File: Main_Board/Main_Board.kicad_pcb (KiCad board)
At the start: 2 copper layers, 3 parts, among them U1 TCR2EF33_LMCT

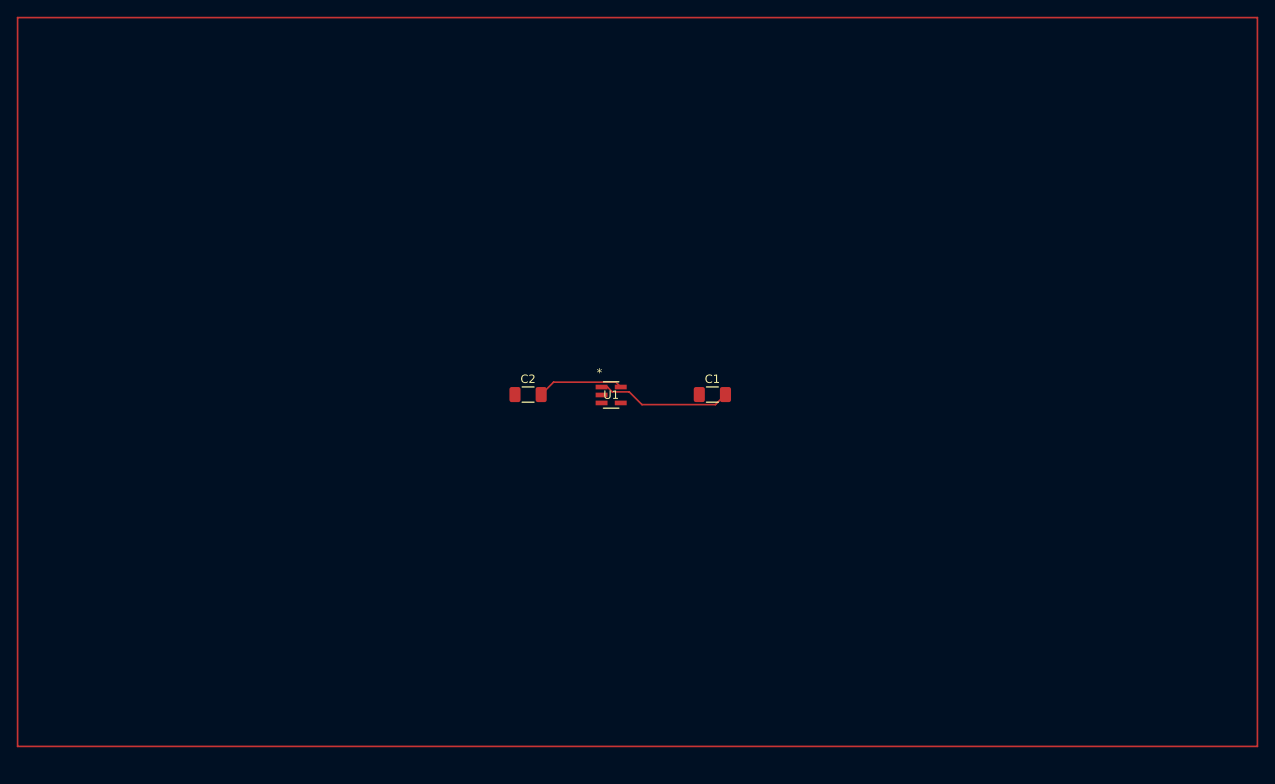
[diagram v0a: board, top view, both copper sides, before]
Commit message: Main board
The schematic is done, tho I have some concerns...
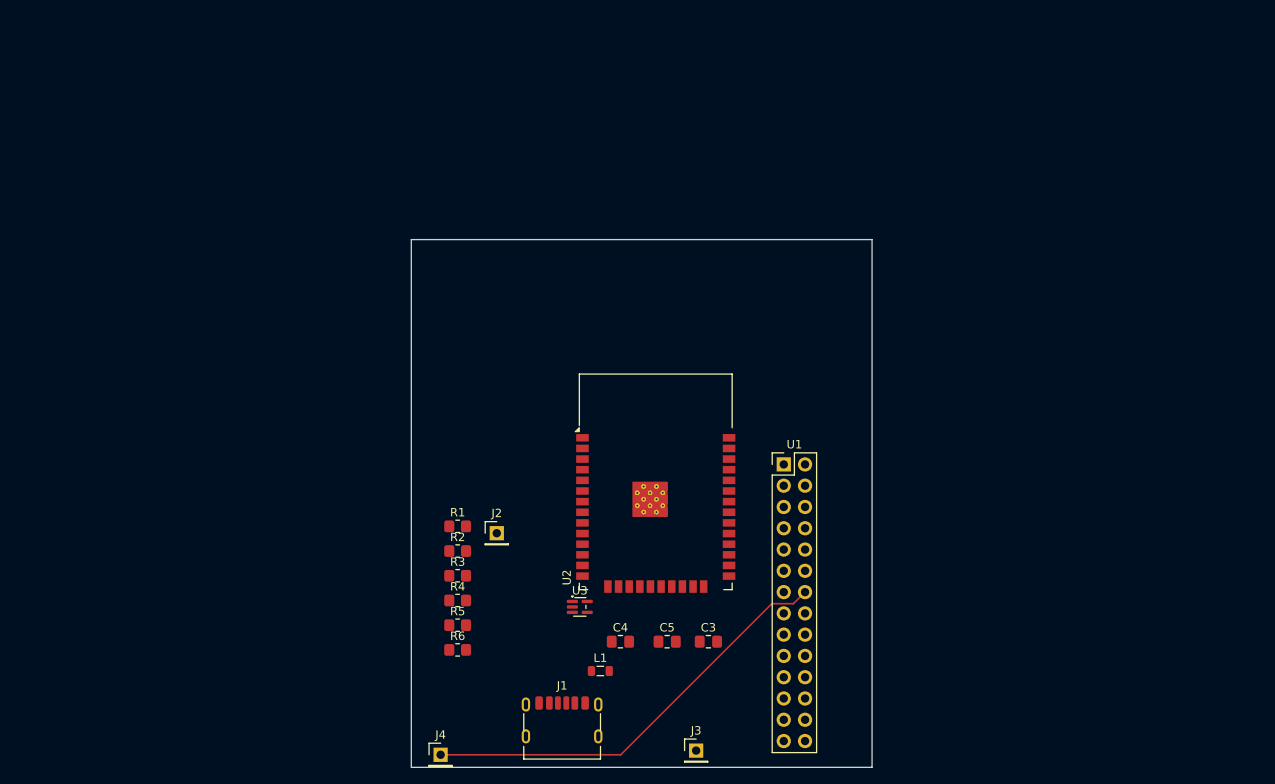
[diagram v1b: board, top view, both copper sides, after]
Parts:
- removed C1, C2: C, Capacitor_SMD:C_1206_3216Metric_Pad1.33x1.80mm_HandSolder
- added C3: 10uF, Capacitor_SMD:C_0805_2012Metric_Pad1.18x1.45mm_HandSolder, F.Cu at (173.5, 136.5)
- added C4: 0.1uF, Capacitor_SMD:C_0805_2012Metric_Pad1.18x1.45mm_HandSolder, F.Cu at (163.0, 136.5)
- added C5: 100uF, Capacitor_SMD:C_0805_2012Metric_Pad1.18x1.45mm_HandSolder, F.Cu at (168.5, 136.5)
- added J1: USB_C_Receptacle_USB2.0_16P, Connector_USB:USB_C_Receptacle_HRO_TYPE-C-31-M-17, F.Cu at (156.0, 147.0)
- added J2: Conn_01x04_Pin, Connector_PinHeader_2.54mm:PinHeader_1x01_P2.54mm_Vertical, F.Cu at (148.2, 123.5)
- added J3: Conn_01x05_Pin, Connector_PinHeader_2.54mm:PinHeader_1x01_P2.54mm_Vertical, F.Cu at (172.0, 149.5)
- added J4: Conn_01x03_Pin, Connector_PinHeader_2.54mm:PinHeader_1x01_P2.54mm_Vertical, F.Cu at (141.5, 150.0)
- added L1: L, Inductor_SMD:L_0805_2012Metric, F.Cu at (160.6, 140.0)
- added R1: 10k, Resistor_SMD:R_0805_2012Metric_Pad1.20x1.40mm_HandSolder, F.Cu at (143.5, 122.7)
- added R2: 10K, Resistor_SMD:R_0805_2012Metric_Pad1.20x1.40mm_HandSolder, F.Cu at (143.5, 125.7)
- added R3: 5.1K, Resistor_SMD:R_0805_2012Metric_Pad1.20x1.40mm_HandSolder, F.Cu at (143.5, 128.6)
- added R4: 5.1K, Resistor_SMD:R_0805_2012Metric_Pad1.20x1.40mm_HandSolder, F.Cu at (143.5, 131.6)
- added R5: 4.7K, Resistor_SMD:R_0805_2012Metric_Pad1.20x1.40mm_HandSolder, F.Cu at (143.5, 134.5)
- added R6: 4.7K, Resistor_SMD:R_0805_2012Metric_Pad1.20x1.40mm_HandSolder, F.Cu at (143.5, 137.5)
- added U2: ESP32-WROOM-32, RF_Module:ESP32-WROOM-32, F.Cu at (167.2, 120.4)
- added U3: TLV9001IDCK, Package_TO_SOT_SMD:SOT-353_SC-70-5, F.Cu at (158.1, 132.3)
- U1: value TCR2EF33_LMCT -> DEV-15583; footprint shared_footprints:SOT-25 SMV_TOS -> Connector_PinHeader_2.54mm:PinHeader_2x14_P2.54mm_Vertical
- moved U1 22.2 mm to (182.5, 115.3)
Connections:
- U1 pad 1: Net-(U1-VIN) -> unconnected-(U1-Pad1)
- U1 pad 5: Net-(U1-VOUT) -> unconnected-(U1-Pad5)
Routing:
- net Net-(J4-Pin_1): track 0.00 -> 51.5 mm
- net Net-(U1-VIN): track 16.2 -> 0.00 mm
- net Net-(U1-VOUT): track 10.4 -> 0.00 mm
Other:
- board outline added: 55 x 63 mm

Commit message: updated main PCB
same thing
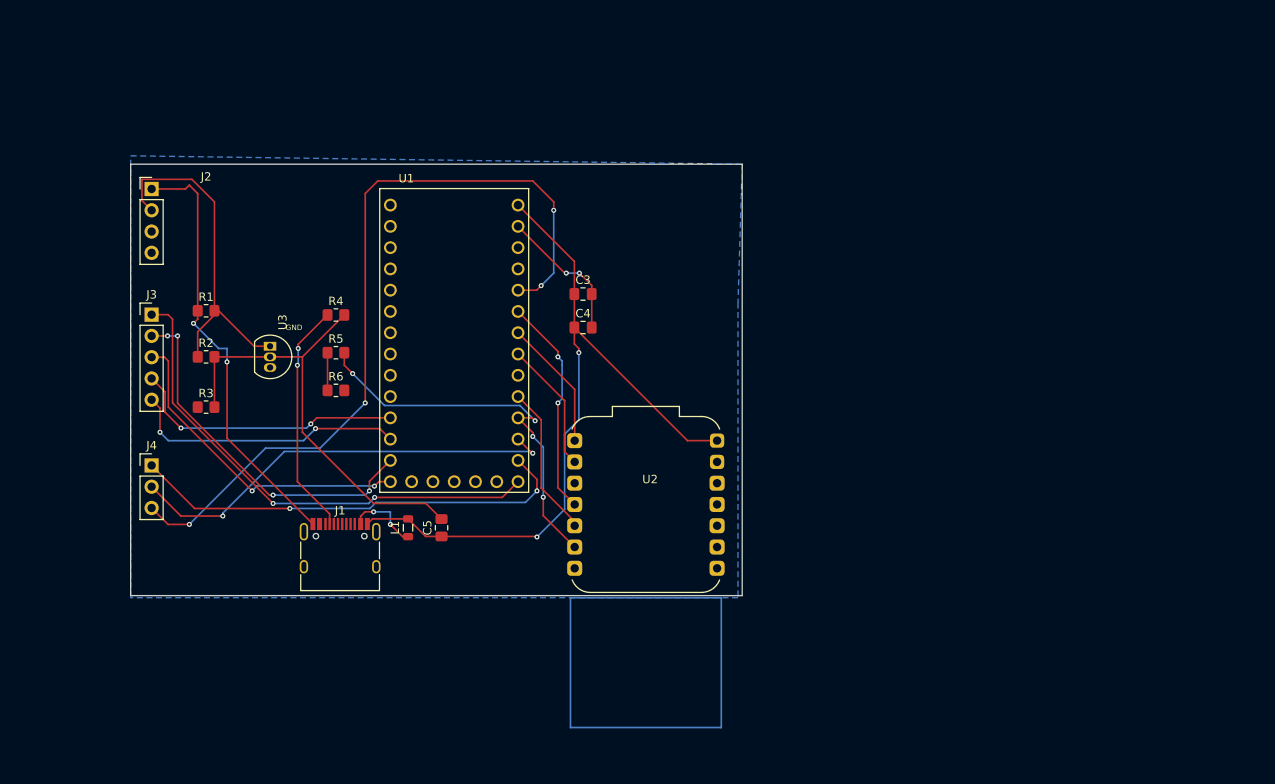
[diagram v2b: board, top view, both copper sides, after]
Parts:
- J1: footprint Connector_USB:USB_C_Receptacle_HRO_TYPE-C-31-M-17 -> Connector_USB:USB_C_Receptacle_HRO_TYPE-C-31-M-12
- J2: footprint Connector_PinHeader_2.54mm:PinHeader_1x01_P2.54mm_Vertical -> Connector_PinHeader_2.54mm:PinHeader_1x04_P2.54mm_Vertical
- J3: footprint Connector_PinHeader_2.54mm:PinHeader_1x01_P2.54mm_Vertical -> Connector_PinHeader_2.54mm:PinHeader_1x05_P2.54mm_Vertical
- J4: footprint Connector_PinHeader_2.54mm:PinHeader_1x01_P2.54mm_Vertical -> Connector_PinHeader_2.54mm:PinHeader_1x03_P2.54mm_Vertical
- U1: footprint Connector_PinHeader_2.54mm:PinHeader_2x14_P2.54mm_Vertical -> shared_footprints:MODULE_DEV-15583
- U2: value ESP32-WROOM-32 -> XIAO-ESP32-C3-DIP; footprint RF_Module:ESP32-WROOM-32 -> RF_Module:MCU_Seeed_ESP32C3
- U3: footprint Package_TO_SOT_SMD:SOT-353_SC-70-5 -> Package_TO_SOT_THT:TO-92_Inline
- moved J3 83.3 mm to (107.0, 97.5)
- moved J2 58.2 mm to (107.0, 82.5)
- moved J4 48.8 mm to (107.0, 115.5)
- moved U3 48.3 mm to (121.1, 101.2), turned to -90 degrees
- moved C3 44.1 mm to (158.5, 95.0)
- moved U1 41.9 mm to (143.1, 100.9)
- moved R1 39.5 mm to (113.5, 97.0)
- moved R2 37.9 mm to (113.5, 102.5)
- moved C4 37.8 mm to (158.5, 99.0)
- moved R4 37.0 mm to (129.0, 97.5)
- moved R3 36.2 mm to (113.5, 108.5)
- moved R5 35.6 mm to (129.0, 102.0)
- moved R6 34.2 mm to (129.0, 106.5)
- moved J1 33.5 mm to (129.5, 126.5)
- moved C5 30.2 mm to (141.6, 122.9), turned to 90 degrees
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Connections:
- R5 pad 2: Net-(U2-IO22) -> Net-(U2-GPIO7/D5/SCL)
- U1 pad 16: Net-(U2-IO22) -> Net-(U2-GPIO7/D5/SCL)
- U1 pad 17: Net-(U2-IO21) -> Net-(U2-GPIO6/D4/SDA)
- U1 pad 18: Net-(U2-SDO/SD0) -> unconnected-(U1-Pad18)
- U1 pad 19: Net-(U2-SENSOR_VN) -> Net-(U2-GPIO3/A1/D1)
- U1 pad 20: Net-(U2-SENSOR_VP) -> Net-(U2-GPIO2/A0/D0)
- U1 pad 21: Net-(U2-EN) -> Net-(U2-GPIO5/A3/D3)
- U2 pad 1: GND -> Net-(U2-GPIO2/A0/D0)
- U2 pad 13: unconnected-(U2-IO14-Pad13) -> GND
- U2 pad 14: unconnected-(U2-IO12-Pad14) -> +5V
- U2 pad 2: unconnected-(U2-VDD-Pad2) -> Net-(U2-GPIO3/A1/D1)
- U2 pad 3: Net-(U2-EN) -> unconnected-(U2-GPIO4/A2/D2-Pad3)
- U2 pad 4: Net-(U2-SENSOR_VP) -> Net-(U2-GPIO5/A3/D3)
- U2 pad 5: Net-(U2-SENSOR_VN) -> Net-(U2-GPIO6/D4/SDA)
- U2 pad 6: unconnected-(U2-IO34-Pad6) -> Net-(U2-GPIO7/D5/SCL)
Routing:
- net +5V: track 0.00 -> 141.0 mm, vias 0 -> 4
- net Net-(J4-Pin_3): track 0.00 -> 95.1 mm, vias 0 -> 4
- net GND: track 0.00 -> 70.2 mm, vias 0 -> 2
- net Net-(J3-Pin_1): track 0.00 -> 60.0 mm, vias 0 -> 2
- net Net-(J4-Pin_2): track 0.00 -> 52.9 mm, vias 0 -> 2
- net Net-(U2-GPIO7/D5/SCL): track 0.00 -> 47.4 mm, vias 0 -> 4
- net Net-(J3-Pin_2): track 0.00 -> 43.5 mm, vias 0 -> 4
- net Net-(J2-Pin_2): track 0.00 -> 41.7 mm
- net Net-(J3-Pin_3): track 0.00 -> 38.8 mm, vias 0 -> 2
- net Net-(J3-Pin_5): track 0.00 -> 33.3 mm, vias 0 -> 2
- net Net-(J3-Pin_4): track 0.00 -> 32.9 mm, vias 0 -> 2
- net Net-(J1-CC1): track 0.00 -> 28.0 mm, vias 0 -> 2
- net Net-(U2-GPIO5/A3/D3): track 0.00 -> 26.3 mm, vias 0 -> 2
- net Net-(U2-GPIO6/D4/SDA): track 0.00 -> 18.2 mm
- net Net-(U2-GPIO3/A1/D1): track 0.00 -> 15.7 mm
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- added copper zone on B.Cu, net GND
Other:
- board size 55 x 63 mm -> 73 x 51.5 mm
